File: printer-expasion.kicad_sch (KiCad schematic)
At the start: 80 parts, among them J1 Screw_Terminal_DC_input, J10 pinda1, J11 pinda2, J12 pinda3, J13 Conn_02x04_Odd_Even, J14 fan, J15 fan, J16 fan, J17 fan, J18 Conn_02x04_Odd_Even, J19 pinda4, J2 motor 1, J3 uart pins, J4 Conn_01x02_Pin, J5 Conn_02x04_Odd_Even, J6 Conn_01x02_Pin, J7 motor 2, J8 Conn_01x02_Pin, J9 motor 3, Q1 NPN, Q2 NPN, Q3 NPN, Q4 NPN, U1 rp2040-zero-pads

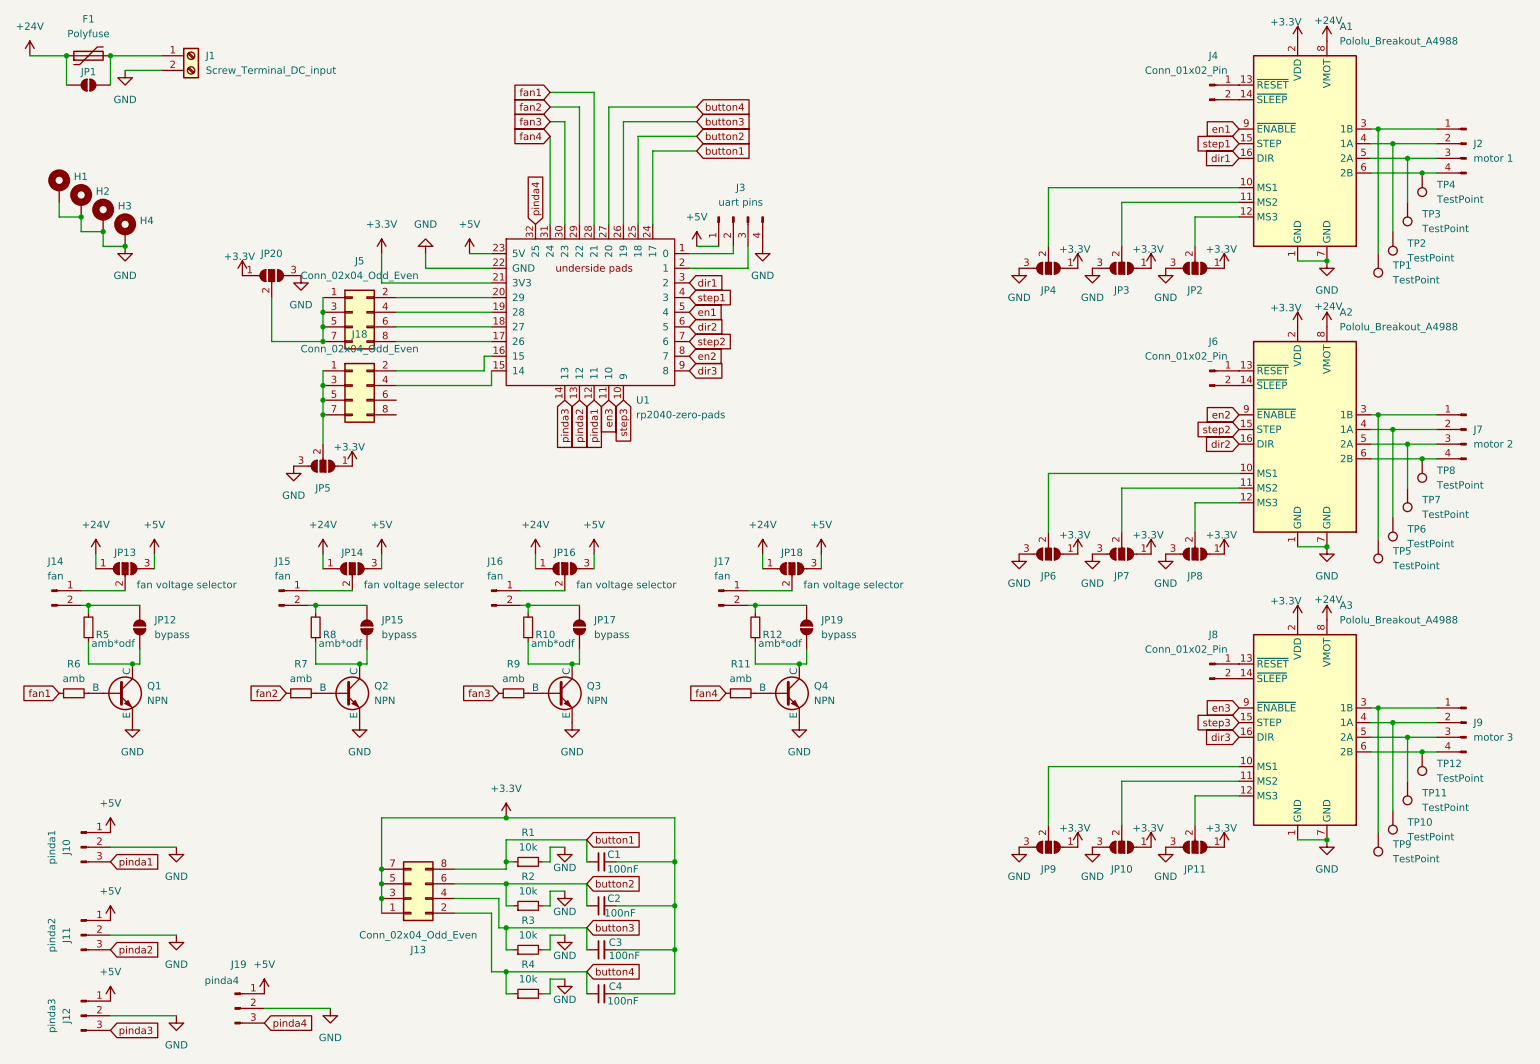
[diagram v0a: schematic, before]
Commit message: final
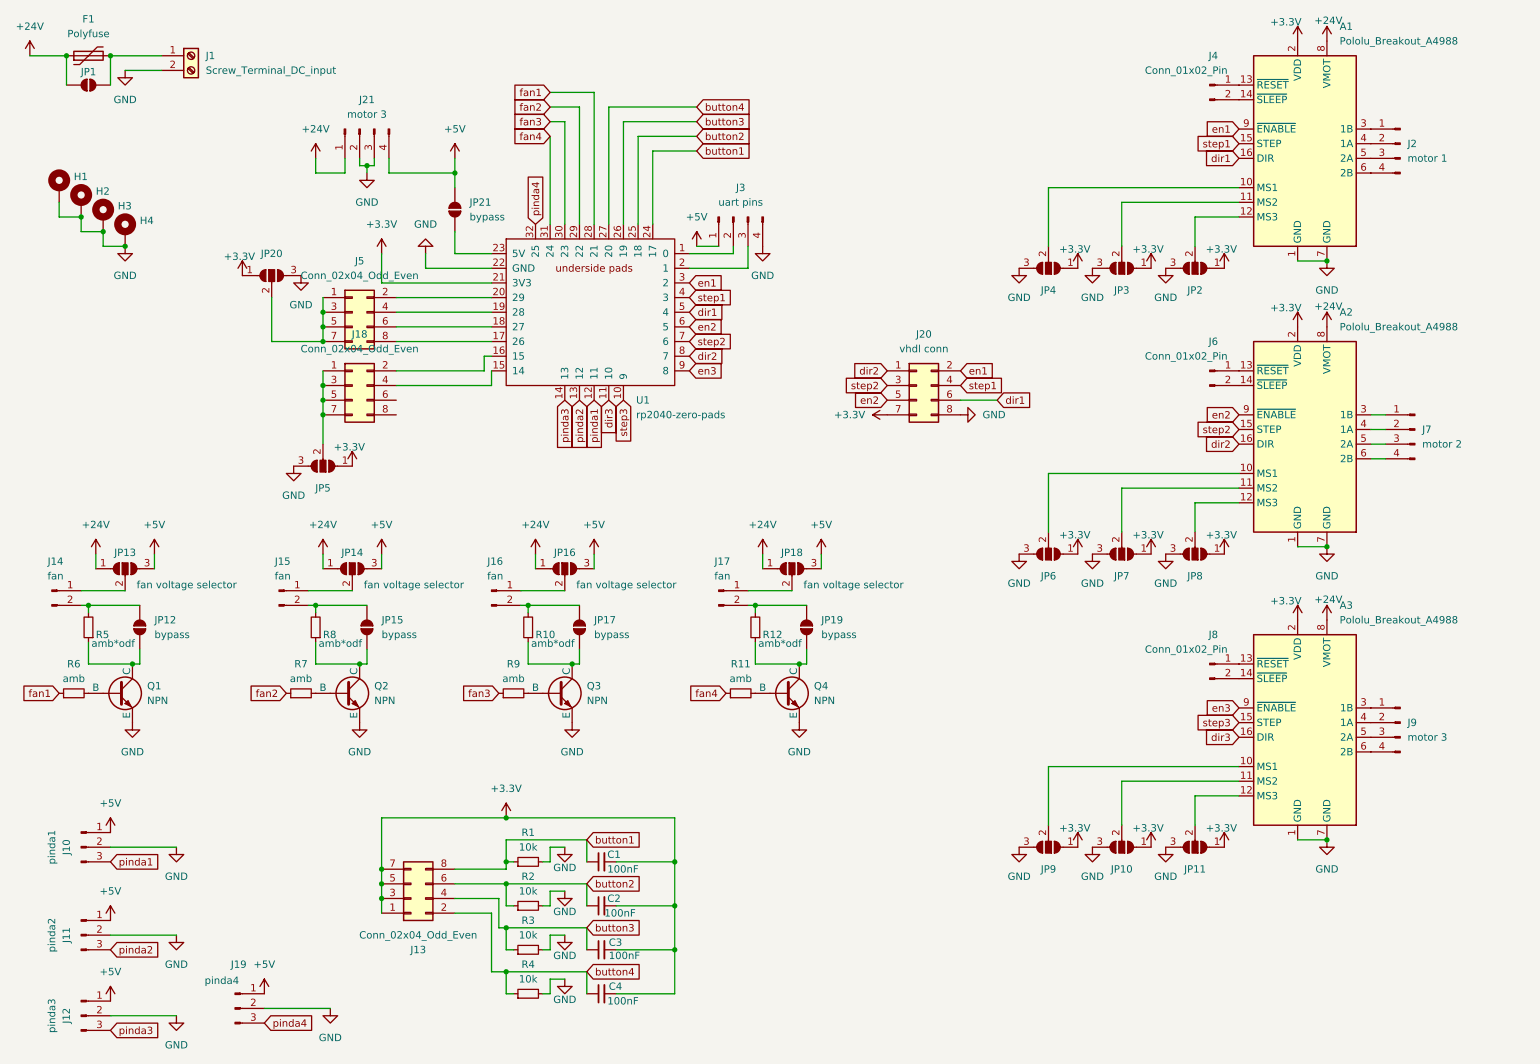
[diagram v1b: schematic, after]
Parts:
- removed TP1, TP10, TP11, TP12, TP2, TP3, TP4, TP5, TP6, TP7, TP8, TP9: TestPoint, TestPoint:TestPoint_THTPad_1.0x1.0mm_Drill0.5mm, symbol Connector:TestPoint
- added J20: vhdl conn, Connector_PinHeader_2.54mm:PinHeader_2x04_P2.54mm_Vertical, symbol Connector_Generic:Conn_02x04_Odd_Even
- added J21: motor 3, Connector_PinHeader_2.54mm:PinHeader_1x04_P2.54mm_Vertical, symbol Connector:Conn_01x04_Pin
- added JP21: bypass, Jumper:SolderJumper-2_P1.3mm_Open_Pad1.0x1.5mm, symbol Jumper:SolderJumper_2_Open
- JP10, JP11, JP2, JP3, JP4, JP6, JP7, JP8, JP9: footprint Jumper:SolderJumper-3_P1.3mm_Open_Pad1.0x1.5mm -> Connector_PinHeader_2.54mm:PinHeader_1x03_P2.54mm_Vertical
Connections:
- net +24V: now also J21.1 (Pin_1)
- net +3.3V: now also J20.7 (Pin_7)
- net +5V: now also J21.4 (Pin_4), JP21.2 (B); no longer U1.23 (5V)
- net GND: now also J20.8 (Pin_8), J21.2 (Pin_2), J21.3 (Pin_3)
- net dir1: now also U1.5 (4), J20.6 (Pin_6); no longer U1.3 (2)
- net dir2: now also U1.8 (7), J20.1 (Pin_1); no longer U1.6 (5)
- net dir3: now also U1.11 (10); no longer U1.9 (8)
- net en1: now also U1.3 (2), J20.2 (Pin_2); no longer U1.5 (4)
- net en2: now also U1.6 (5), J20.5 (Pin_5); no longer U1.8 (7)
- net en3: now also U1.9 (8); no longer U1.11 (10)
- net step1: now also J20.4 (Pin_4)
- net step2: now also J20.3 (Pin_3)
- new net: JP21.1 (A), U1.23 (5V)
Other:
- moved on the sheet: J2, J7, J9
